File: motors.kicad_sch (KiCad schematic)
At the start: 29 parts, among them Q1 NMOS, Q2 NMOS, Q3 NMOS, Q4 NMOS, U16 DRV8328ARUYR

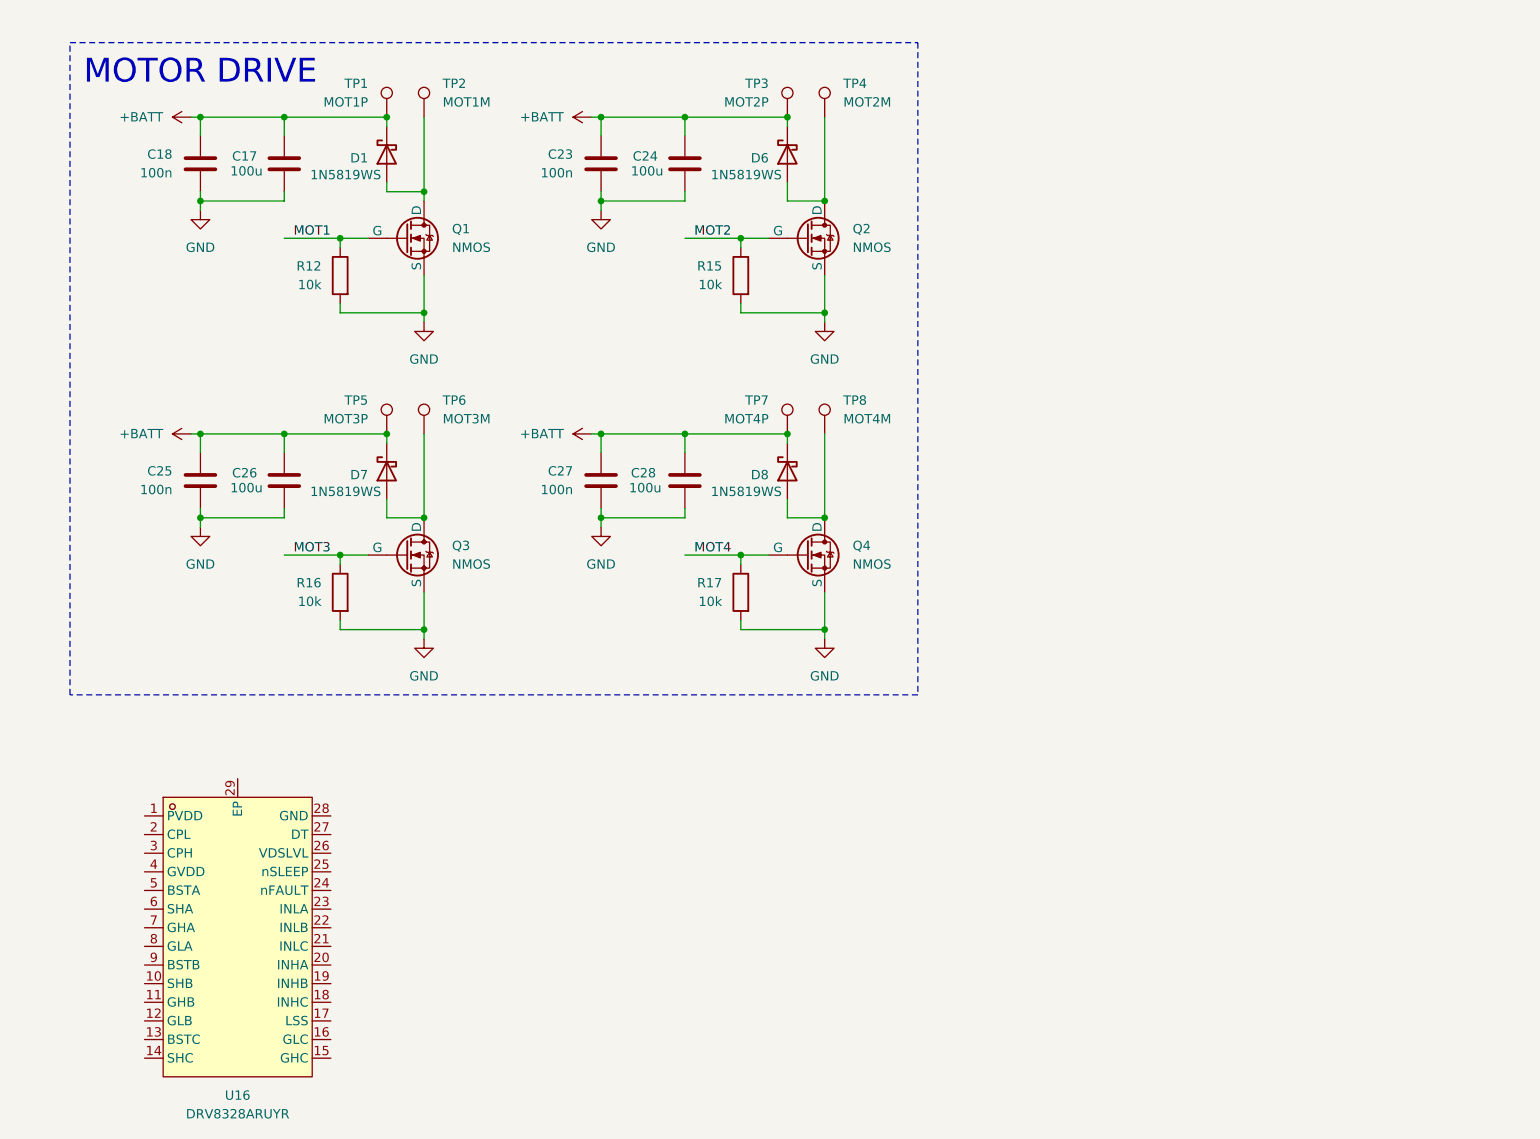
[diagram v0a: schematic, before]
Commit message: Restore all functionality from v1
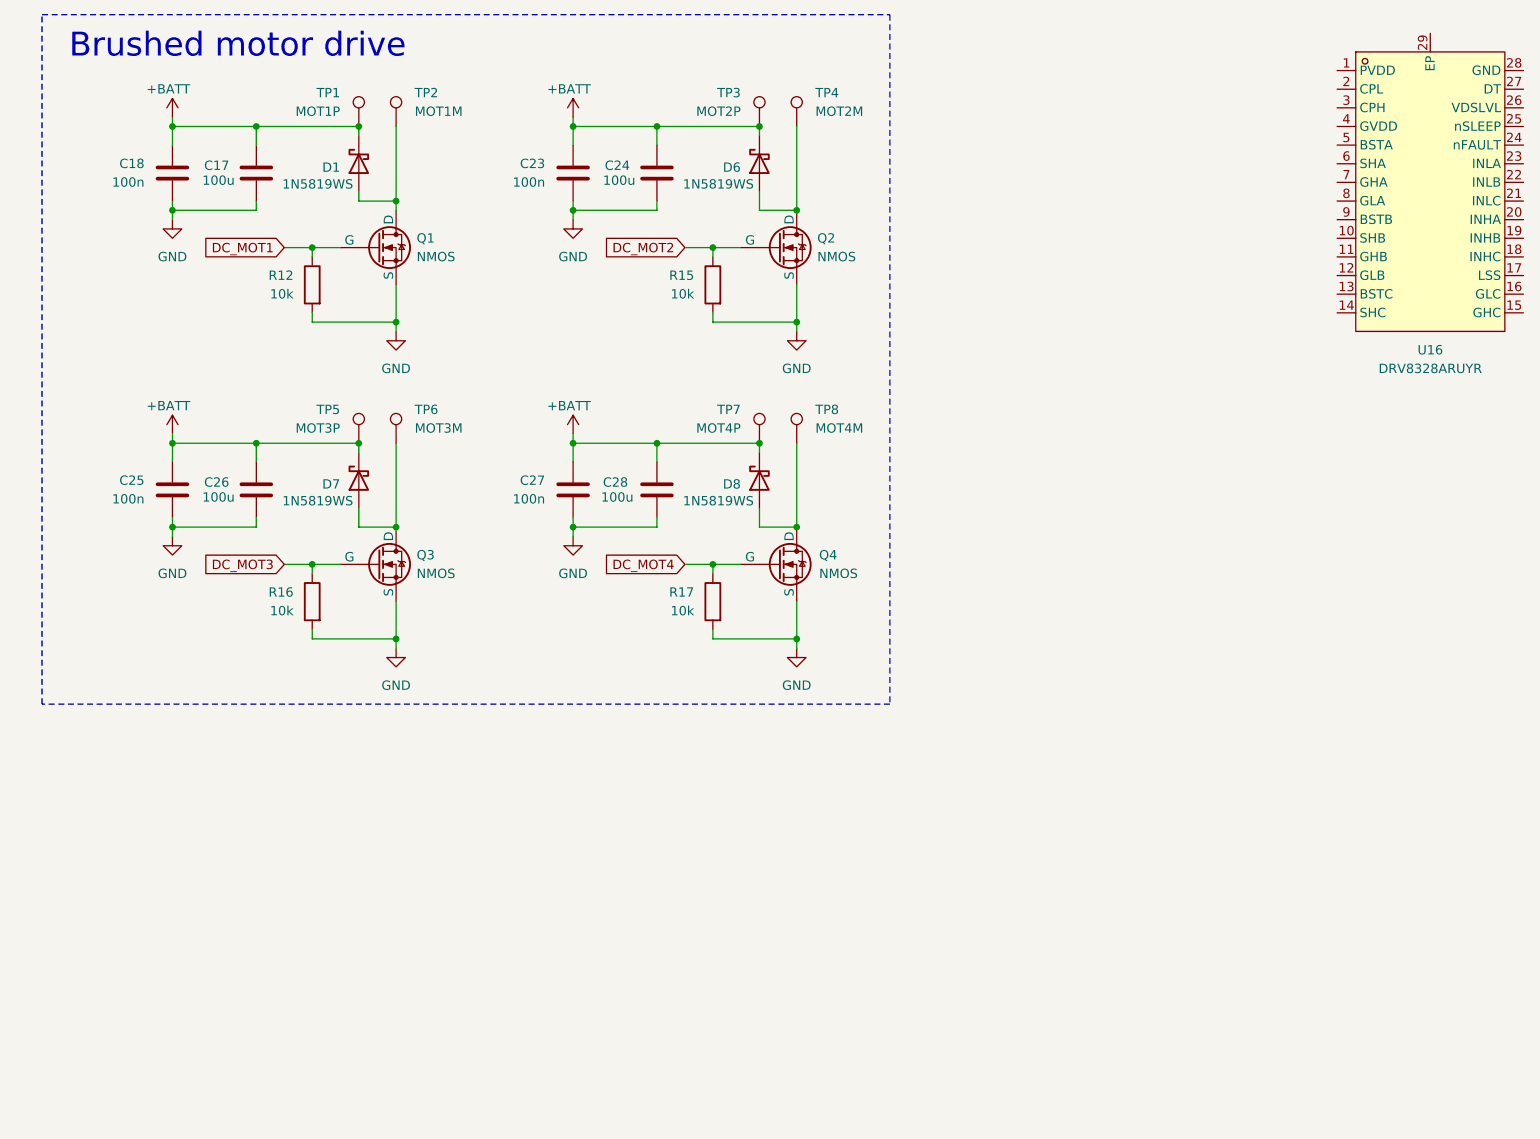
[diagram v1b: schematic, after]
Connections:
- net MOT1 renamed DC_MOT1
- net MOT2 renamed DC_MOT2
- net MOT3 renamed DC_MOT3
- net MOT4 renamed DC_MOT4
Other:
- note added: "Brushed motor drive"
- note removed: "MOTOR DRIVE"
- moved on the sheet: C17, C18, C23, C24, C25, C26, C27, C28, D1, D6, D7, D8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
